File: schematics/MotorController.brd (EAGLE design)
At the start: 120.6 x 92.4 mm, 36 parts, among them IC1 7805, K1 35701331, T1 BC338

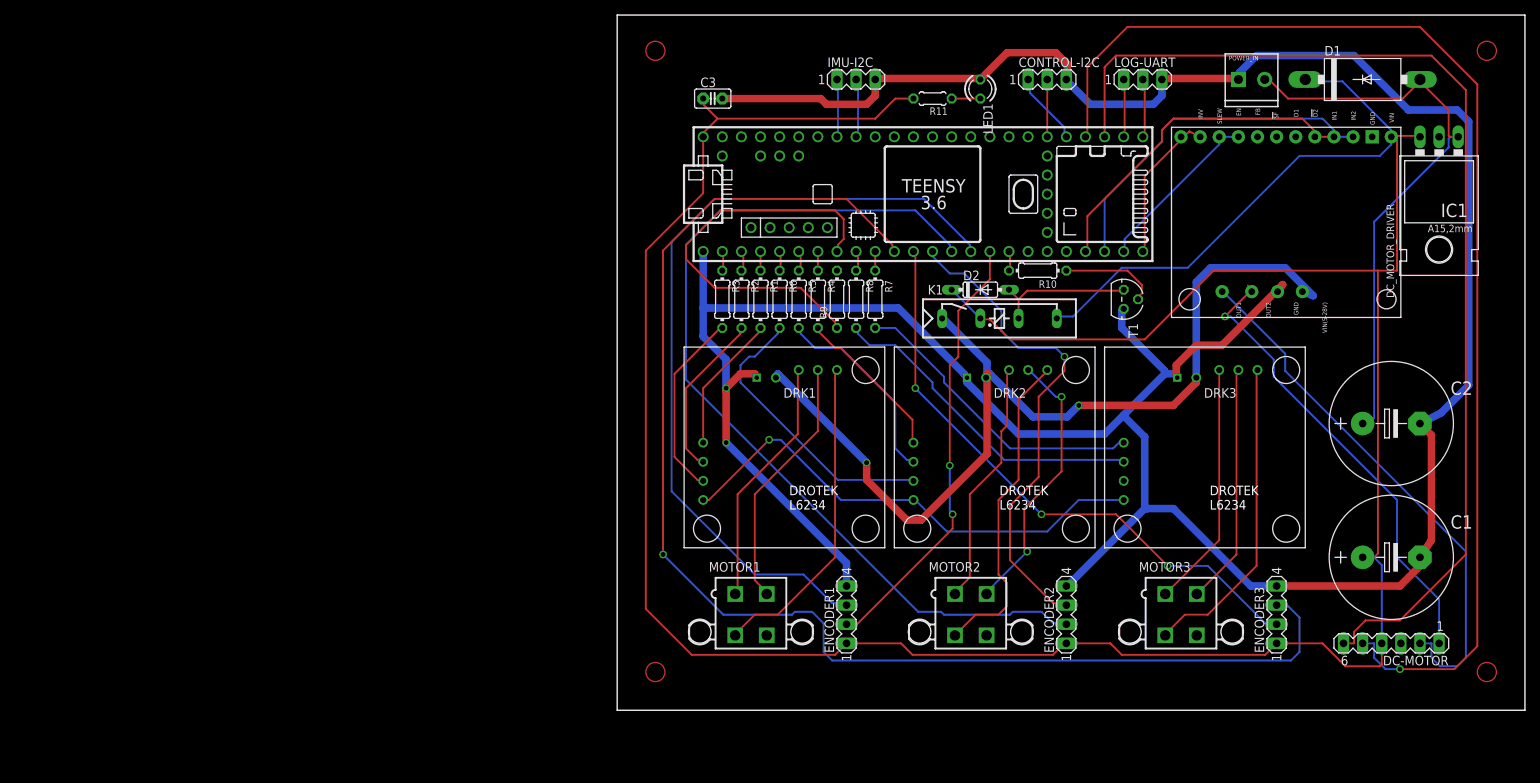
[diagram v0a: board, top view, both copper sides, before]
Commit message: no message
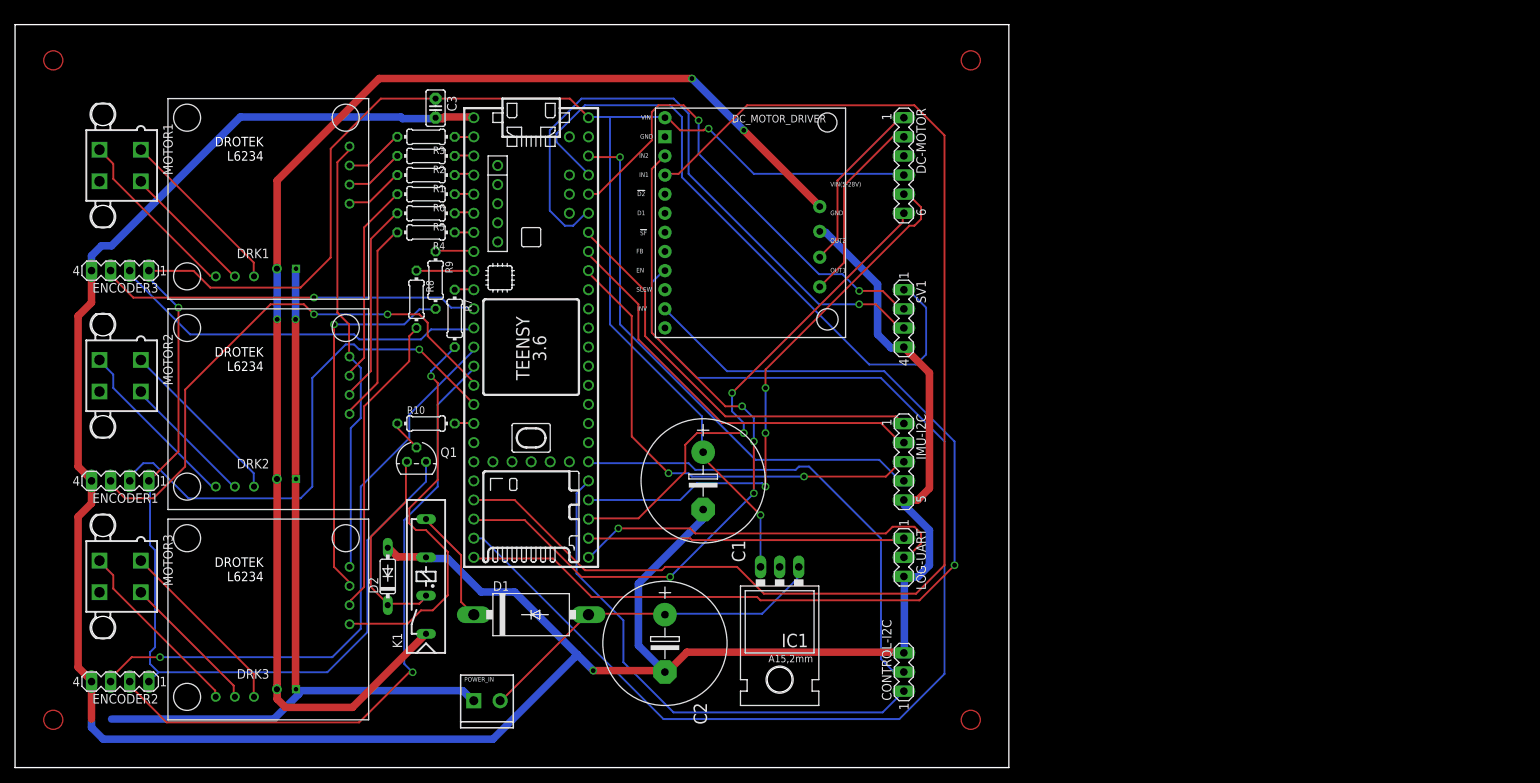
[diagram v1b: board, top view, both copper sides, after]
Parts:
- removed LED1: green, led:LED3MM
- removed R11: 1K, resistor:0204/5
- removed T1: BC338, transistor:TO92
- added Q1: BC307, transistor-pnp:TO92
- added SV1: (no value), con-lstb:MA04-1
- IMU-I2C: device con-lstb:MA03-1 -> con-lstb:MA05-1
- moved ENCODER3 160.3 mm to (-58.4, 57.1), turned to 180 degrees
- moved MOTOR3 141.1 mm to (-58.4, 16.5), turned to 90 degrees
- moved D1 131.4 mm to (-3.81, 11.4)
- moved POWER_IN 130.9 mm to (-11.4, 0.00)
- moved DRK3 127.6 mm to (-39.4, 11.4), turned to 180 degrees
- moved ENCODER2 126.0 mm to (-58.4, 2.54), turned to 180 degrees
- moved MOTOR2 117.4 mm to (-58.4, 43.2), turned to 90 degrees
- moved IC1 104.6 mm to (29.2, 14.0)
- moved MOTOR1 102.9 mm to (-58.4, 71.1), turned to 90 degrees
- moved C2 100.8 mm to (14.0, 7.62), turned to 270 degrees
- moved ENCODER1 98.1 mm to (-58.4, 29.2), turned to 180 degrees
- moved DRK2 98.0 mm to (-39.4, 39.4), turned to 180 degrees
- moved C1 92.0 mm to (19.1, 29.2), turned to 270 degrees
- moved DC-MOTOR 90.7 mm to (45.7, 71.1), turned to 270 degrees
- moved D2 87.5 mm to (-22.9, 16.5), turned to 90 degrees
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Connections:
- removed net N$40: LED1.K, R11.1
- new net N$46: IMU-I2C.4, PRJ1.3V3_LO
- new net N$48: IMU-I2C.1, PRJ1.20/A6
- new net N$49: PRJ1.23/A9, SV1.1
- new net N$50: PRJ1.22/A8, SV1.2
- new net N$51: PRJ1.21/A7, SV1.3
- net GND: now also D2.A, IMU-I2C.5, K1.5, SV1.4; no longer IMU-I2C.3, LED1.A, T1.1
- net IMU-SCL: now also IMU-I2C.2; no longer IMU-I2C.1
- net IMU-SDA: now also IMU-I2C.3; no longer IMU-I2C.2
- net N$30: now also Q1.2; no longer T1.2
- net N$31: now also D2.C, K1.3, Q1.3; no longer D2.A, K1.5, T1.3
- net VCC: now also Q1.1; no longer D2.C, K1.3, R11.2
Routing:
- net N$45: track 22.9 -> 159.8 mm
- net N$33: track 179.1 -> 50.8 mm
- net N$44: track 44.9 -> 169.5 mm
- net N$41: track 20.2 -> 130.4 mm, vias 0 -> 1
- net N$49: track 0.00 -> 87.6 mm
- net Y_ENC_A: track 160.3 -> 73.8 mm, vias 1 -> 3
- net N$51: track 0.00 -> 83.5 mm, vias 0 -> 1
- net WH_ENC_B: track 143.6 -> 66.8 mm, vias 0 -> 2
- net N$46: track 0.00 -> 72.8 mm, vias 0 -> 1
- net N$50: track 0.00 -> 62.8 mm, vias 0 -> 2
- net GND: track 413.9 -> 474.3 mm
- net CTRL-SDA: track 9.78 -> 68.5 mm
- net N$48: track 0.00 -> 56.2 mm
- net IMU-SDA: track 7.88 -> 63.7 mm, vias 0 -> 2
- net N$43: track 7.62 -> 63.2 mm
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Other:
- board size 120.6 x 92.4 mm -> 132.1 x 98.7 mm

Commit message: no message
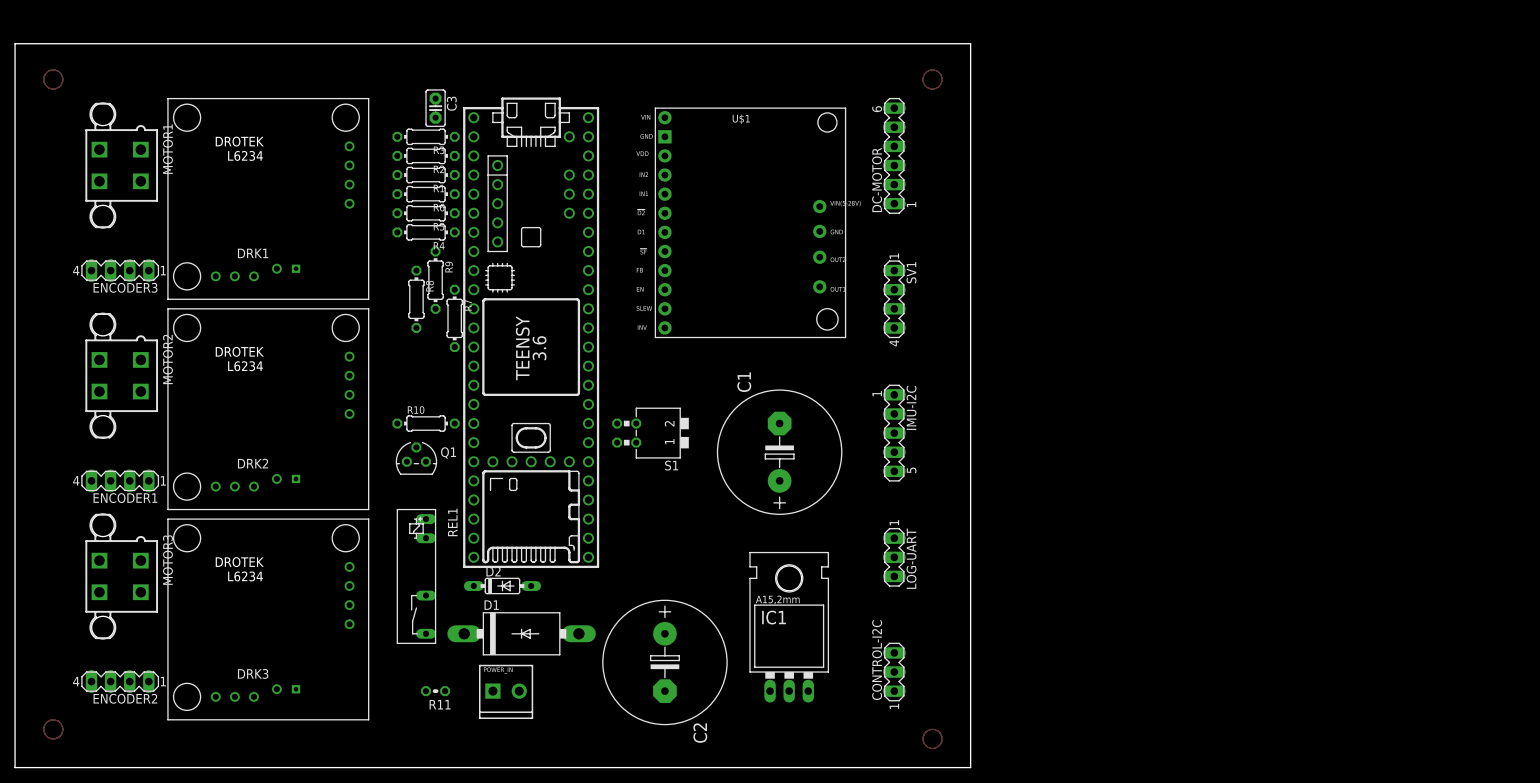
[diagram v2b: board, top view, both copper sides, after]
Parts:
- removed K1: 35701331, relay:REED
- added R11: 0, resistor:0204V
- added REL1: HF49FD, relay:HF49FD
- added S1: (no value), switch-dil:DA-02
- moved D2 15.3 mm to (-7.62, 15.2), turned to 0 degrees
- moved C1 10.9 mm to (29.2, 33.0), turned to 90 degrees
- moved IC1 8.98 mm to (30.5, 5.08), turned to 0 degrees
- moved IMU-I2C 4.02 mm to (44.5, 35.6)
- moved SV1 2.84 mm to (44.5, 53.3)
- moved D1 2.84 mm to (-5.08, 8.89)
- moved POWER_IN 2.84 mm to (-8.89, 1.27)
- moved C2 2.54 mm to (14.0, 5.08)
- moved DC-MOTOR 1.80 mm to (44.5, 72.4), turned to 90 degrees
- moved CONTROL-I2C 1.27 mm to (44.5, 3.81)
- moved LOG-UART 1.27 mm to (44.5, 19.1)
- renumbered DC_MOTOR_DRIVER to U$1
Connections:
- new net LIPO-GND: DRK1.GND, DRK2.GND, DRK3.GND, POWER_IN.1, R11.1, U$1.GND
- new net LIPO-VDD: DRK1.LIPO+, DRK2.LIPO+, DRK3.LIPO+, REL1.3, U$1.VIN(5-28V)
- new net N$40: PRJ1.39/A20, S1.4
- net BLCK-M2: now also U$1.OUT2; no longer U$1.OUT1
- net GND: now also R11.2, REL1.2, S1.1, S1.2; no longer DRK1.GND, DRK2.GND, DRK3.GND, K1.5, POWER_IN.1, U$1.GND
- net N$12: now also PRJ1.21/DAC0, S1.3; no longer DRK1.LIPO+, DRK2.LIPO+, DRK3.LIPO+, K1.1, U$1.VIN(5-28V)
- net N$31: now also REL1.1; no longer K1.3
- net N$39: now also REL1.4; no longer K1.7
- net N$41: now also U$1.VDD; no longer U$1.INV
- net RED-M1: now also U$1.OUT1; no longer U$1.OUT2
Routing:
- net GND: track 474.3 -> 0.00 mm, vias 2 -> 0
- net VCC: track 308.2 -> 0.00 mm, vias 3 -> 0
- net N$12: track 178.0 -> 0.00 mm, vias 3 -> 0
- net N$44: track 169.5 -> 0.00 mm
- net N$45: track 159.8 -> 0.00 mm
- net N$41: track 130.4 -> 0.00 mm, vias 1 -> 0
- net N$47: track 97.5 -> 0.00 mm, vias 4 -> 0
- net N$36: track 87.9 -> 0.00 mm, vias 1 -> 0
- net N$49: track 87.6 -> 0.00 mm
- net N$51: track 83.5 -> 0.00 mm, vias 1 -> 0
- net N$35: track 80.1 -> 0.00 mm, vias 1 -> 0
- net Y_ENC_A: track 73.8 -> 0.00 mm, vias 3 -> 0
- net N$46: track 72.8 -> 0.00 mm, vias 1 -> 0
- net N$37: track 71.9 -> 0.00 mm, vias 2 -> 0
- net N$38: track 69.2 -> 0.00 mm, vias 1 -> 0
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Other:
- board size 132.1 x 98.7 mm -> 127 x 96.2 mm
